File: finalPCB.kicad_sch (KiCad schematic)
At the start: 69 parts, among them J1 9V Battery, J2 FCR7350R, J3 FCR7350R, J4 FCR7350R, J5 Switch, K1 HFD4/005, K2 HFD4/005, K3 HFD4/005, Q1 IRLML6401, Q2 IRLML6401, Q3 IRLML6401, Q4 IRLML6401, Q5 IRLML6401, Q6 NMOS, SW1 SW_Omron_B3FS, SW2 SW_Omron_B3FS, U1 7414, U1 ACS723xLCTR-05AB, U1 LMV358, U2 LMV358, U5 L7805

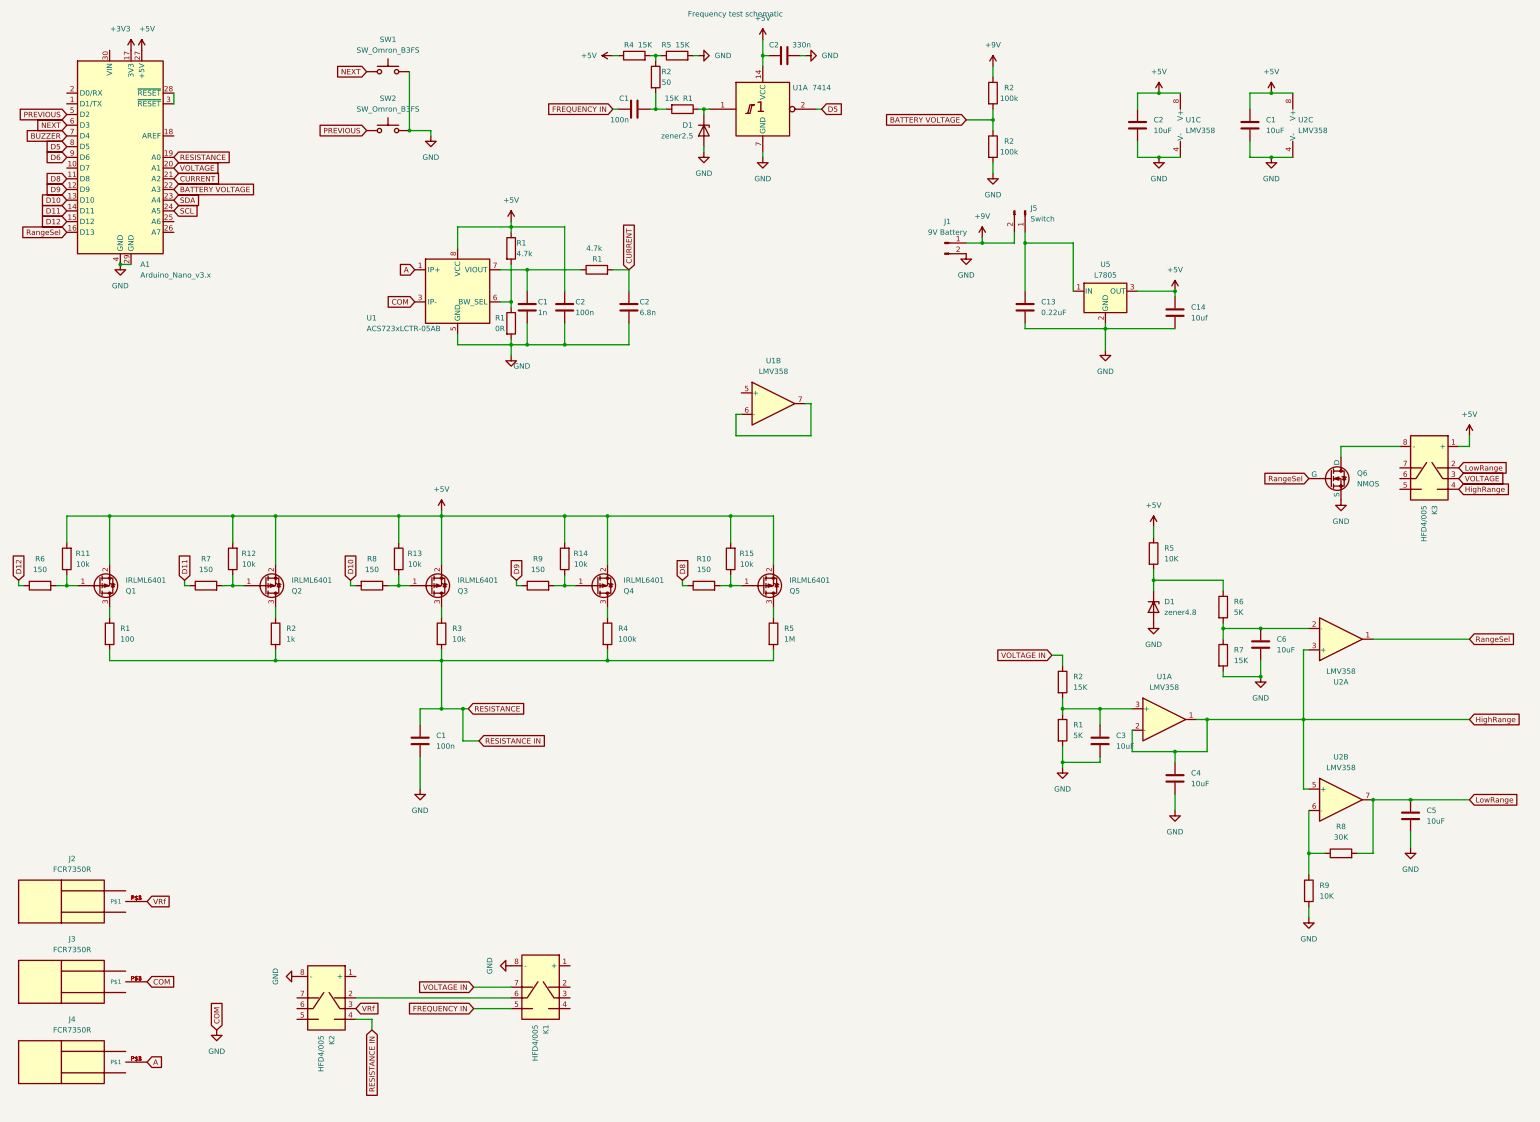
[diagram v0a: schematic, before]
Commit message: V0.1 Done
The first full routing is complete. There is no LM35 sensor included.

PS.
The silkscreen art can be removed, but please no;)
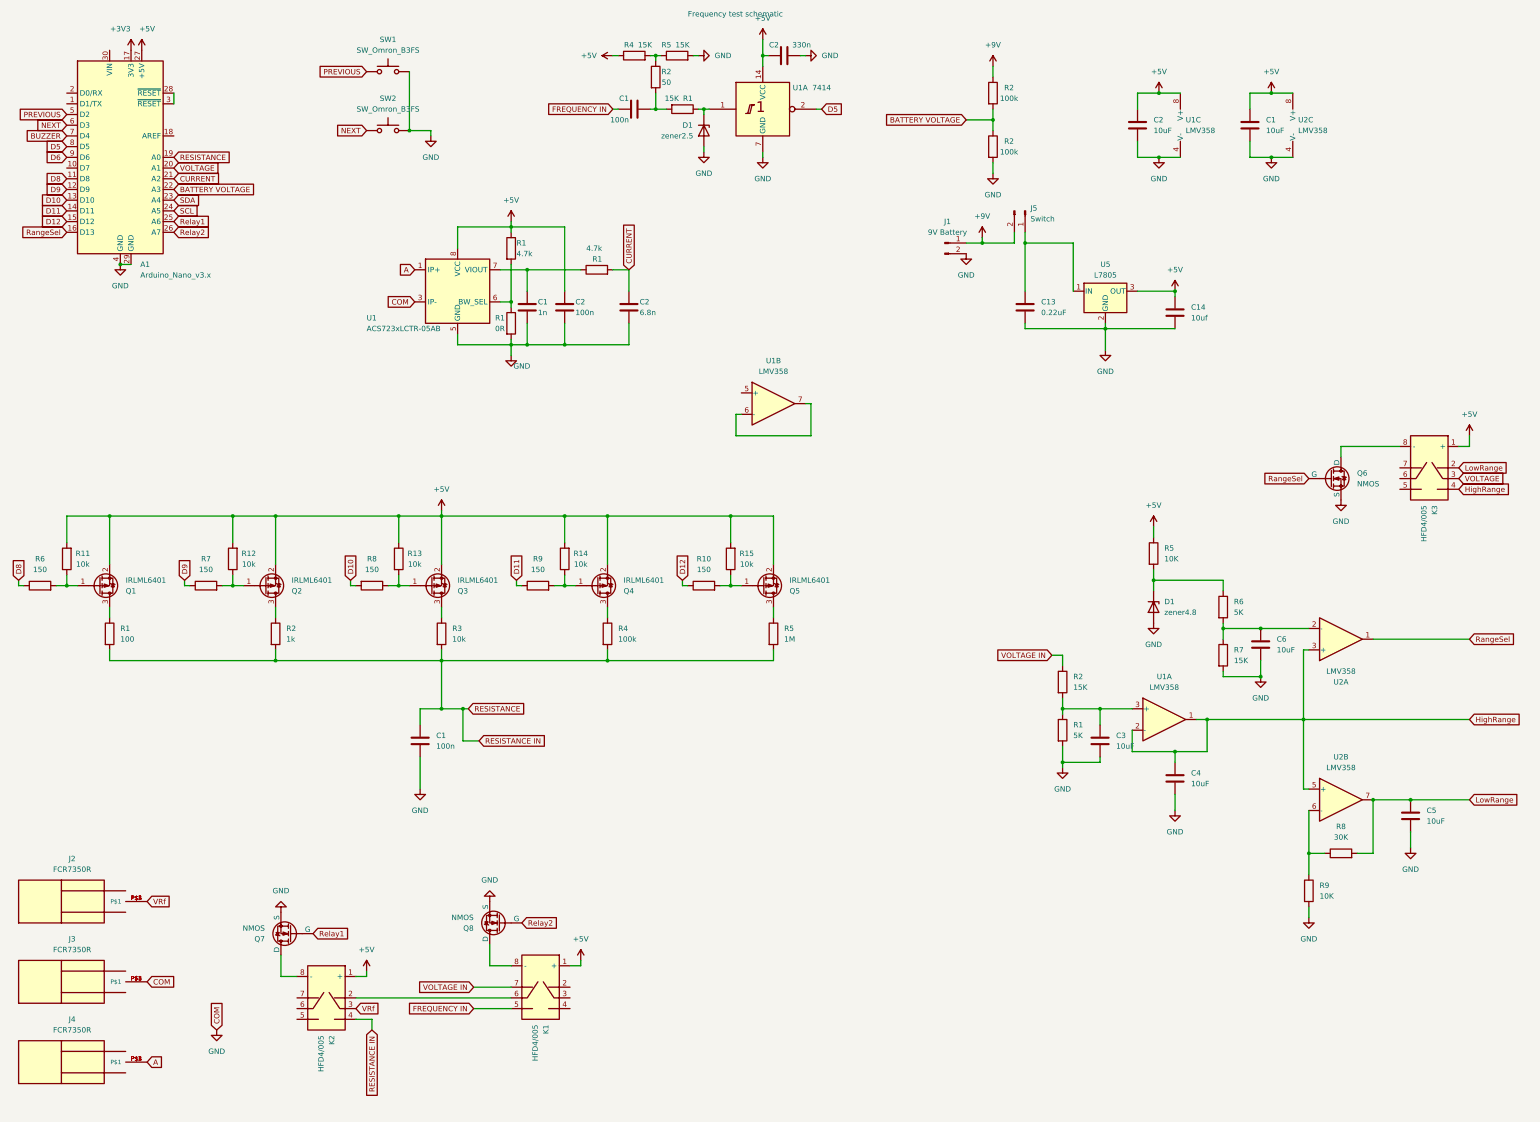
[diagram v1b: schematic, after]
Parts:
- added Q7, Q8: NMOS, Package_TO_SOT_SMD:SOT-23-3, symbol Simulation_SPICE:NMOS
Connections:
- net +5V: now also K1.1 (+), K2.1 (+)
- net D11: now also R9.1; no longer R7.1
- net D12: now also R10.1; no longer R6.1
- net D8: now also R6.1; no longer R10.1
- net D9: now also R7.1; no longer R9.1
- net GND: now also Q7.3 (S), Q8.3 (S); no longer K1.8 (-), K2.8 (-)
- net NEXT: now also SW2.1; no longer SW1.1
- net PREVIOUS: now also SW1.1; no longer SW2.1
- net Relay1: now reaches A1.25 (A6)
- net Relay1: now also Q7.2 (G)
- net Relay2: now reaches A1.26 (A7)
- net Relay2: now also Q8.2 (G)
- new net: K1.8 (-), Q8.1 (D)
- new net: K2.8 (-), Q7.1 (D)
